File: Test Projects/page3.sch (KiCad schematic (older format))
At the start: 1 part, among them U2 Teensy_3.2

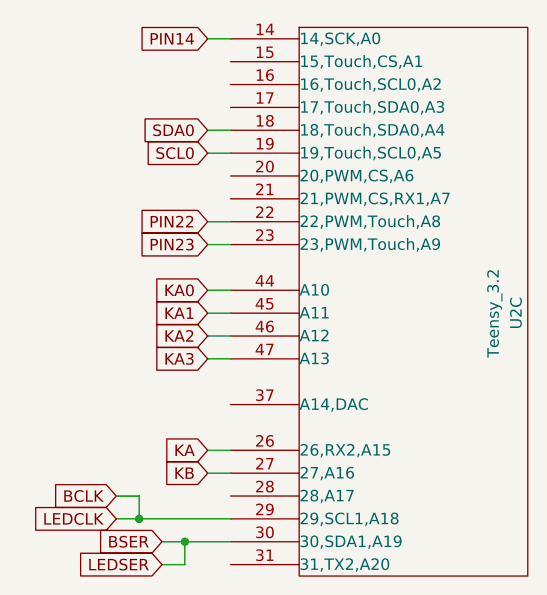
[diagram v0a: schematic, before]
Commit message: Tested a few layout sections
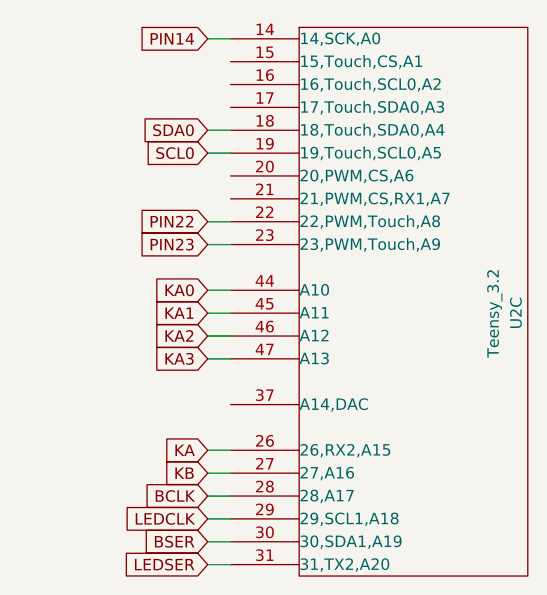
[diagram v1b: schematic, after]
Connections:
- net BCLK: now also U2.28 (28,A17); no longer U2.29 (29,SCL1,A18)
- net LEDSER: now reaches U2.31 (31,TX2,A20)
- new net LEDCLK: U2.29 (29,SCL1,A18)
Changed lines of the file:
@@
 Wire Wire Line
 	4950 4800 4850 4800
-Text GLabel 4650 5100 0    50   Input ~ 0
+Text GLabel 4850 5100 0    50   Input ~ 0
 BSER
-Text GLabel 4650 5200 0    50   Input ~ 0
+Text GLabel 4850 5200 0    50   Input ~ 0
 LEDSER
-Text GLabel 4450 5000 0    50   Input ~ 0
+Text GLabel 4850 5000 0    50   Input ~ 0
 LEDCLK
-Text GLabel 4450 4900 0    50   Input ~ 0
+Text GLabel 4850 4900 0    50   Input ~ 0
 BCLK
 Wire Wire Line
-	4450 5000 4950 5000
+	4850 5000 4950 5000
 Wire Wire Line
-	4550 5000 4550 4900
+	4850 5100 4950 5100
 Wire Wire Line
-	4650 5100 4950 5100
+	4950 5200 4850 5200
 Wire Wire Line
-	4750 5200 4650 5200
-Connection ~ 4750 5100
-Wire Wire Line
-	4550 4900 4450 4900
-Connection ~ 4550 5000
-Wire Wire Line
-	4750 5200 4750 5100
+	4950 4900 4850 4900
 $EndSCHEMATC
